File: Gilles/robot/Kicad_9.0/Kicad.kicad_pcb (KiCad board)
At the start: 2 copper layers, 60 x 34 mm, 10 parts, among them J1 XH2.54_2P_socket, J2 XH2.54_2P_socket, J3 XH2.54_2P_socket, J4 Conn_01x04_Socket, SW1 SW_MINI_x1, U1 ESP32-C3_SUPERMINI, U2 L293D

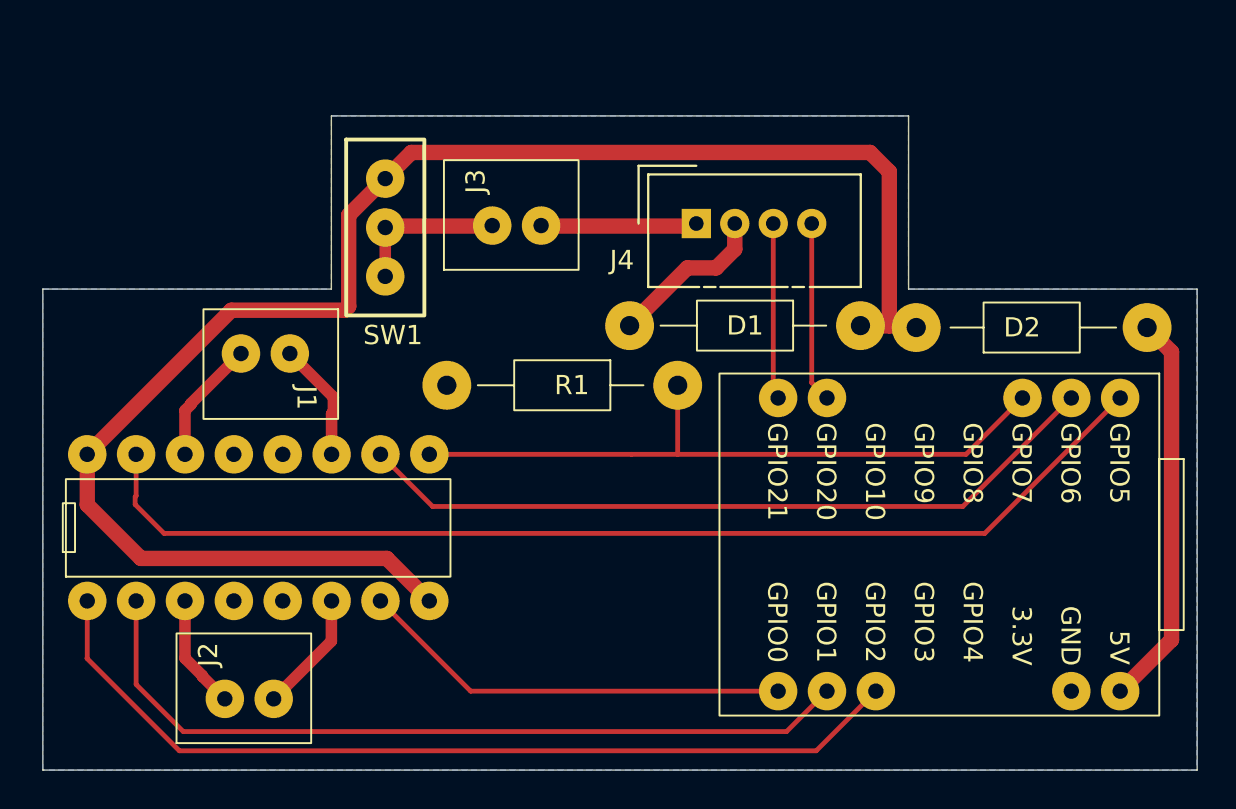
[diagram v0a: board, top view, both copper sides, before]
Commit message: Add files via upload
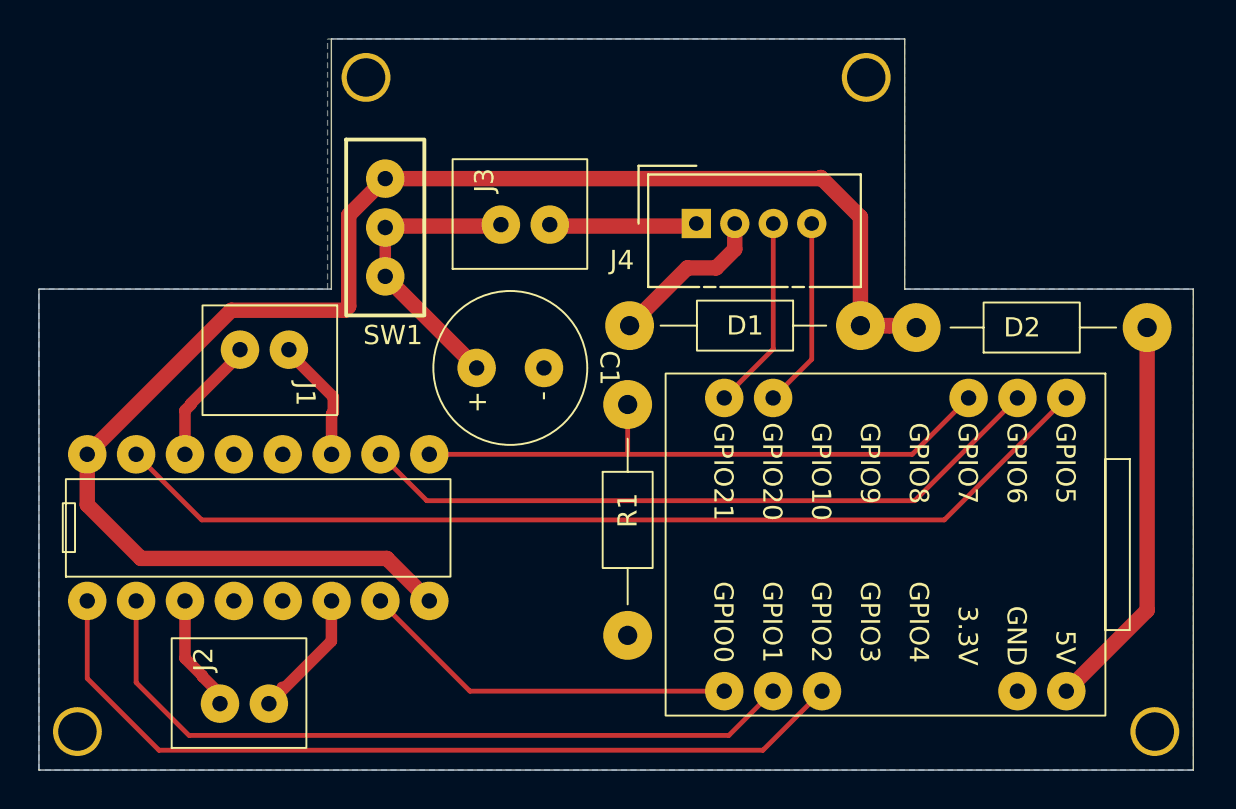
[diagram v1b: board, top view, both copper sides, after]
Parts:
- added C1: C_Polarized, Gilles_Library:CP_8mm_3.5mm, F.Cu at (193.8, 64.1)
- added DH1: DRILL, Gilles_Library:DRILL_HOLE, F.Cu at (188.0, 49.0)
- added DH2: DRILL, Gilles_Library:DRILL_HOLE, F.Cu at (214.0, 49.0)
- added DH3: DRILL, Gilles_Library:DRILL_HOLE, F.Cu at (173.0, 83.0)
- added DH4: DRILL, Gilles_Library:DRILL_HOLE, F.Cu at (229.0, 83.0)
- moved R1 7.78 mm to (201.6, 72.0), turned to 0 degrees
- moved U1 2.80 mm to (215.5, 73.3)
- moved J3 0.45 mm to (197.6, 56.6)
- moved J2 0.35 mm to (182.9, 81.5)
- moved J1 0.21 mm to (181.4, 63.1)
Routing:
- net Net-(SW1-B): track 8.08 -> 14.8 mm
- net Net-(U1-GPIO5): track 57.4 -> 52.4 mm
- net Net-(SW1-A): track 87.6 -> 83.6 mm
- net Net-(U1-GPIO7): track 35.6 -> 31.8 mm
- net Net-(U1-GPIO6): track 39.4 -> 36.3 mm
- net Net-(U1-GPIO0): track 22.6 -> 19.8 mm
- net Net-(U1-GPIO1): track 42.1 -> 39.4 mm
- net Net-(U1-GPIO2): track 47.3 -> 45.0 mm
- net Net-(J4-Pin_4): track 9.40 -> 10.9 mm
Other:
- board size 60 x 34 mm -> 60 x 38 mm
